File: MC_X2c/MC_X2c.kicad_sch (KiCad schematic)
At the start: 0 parts

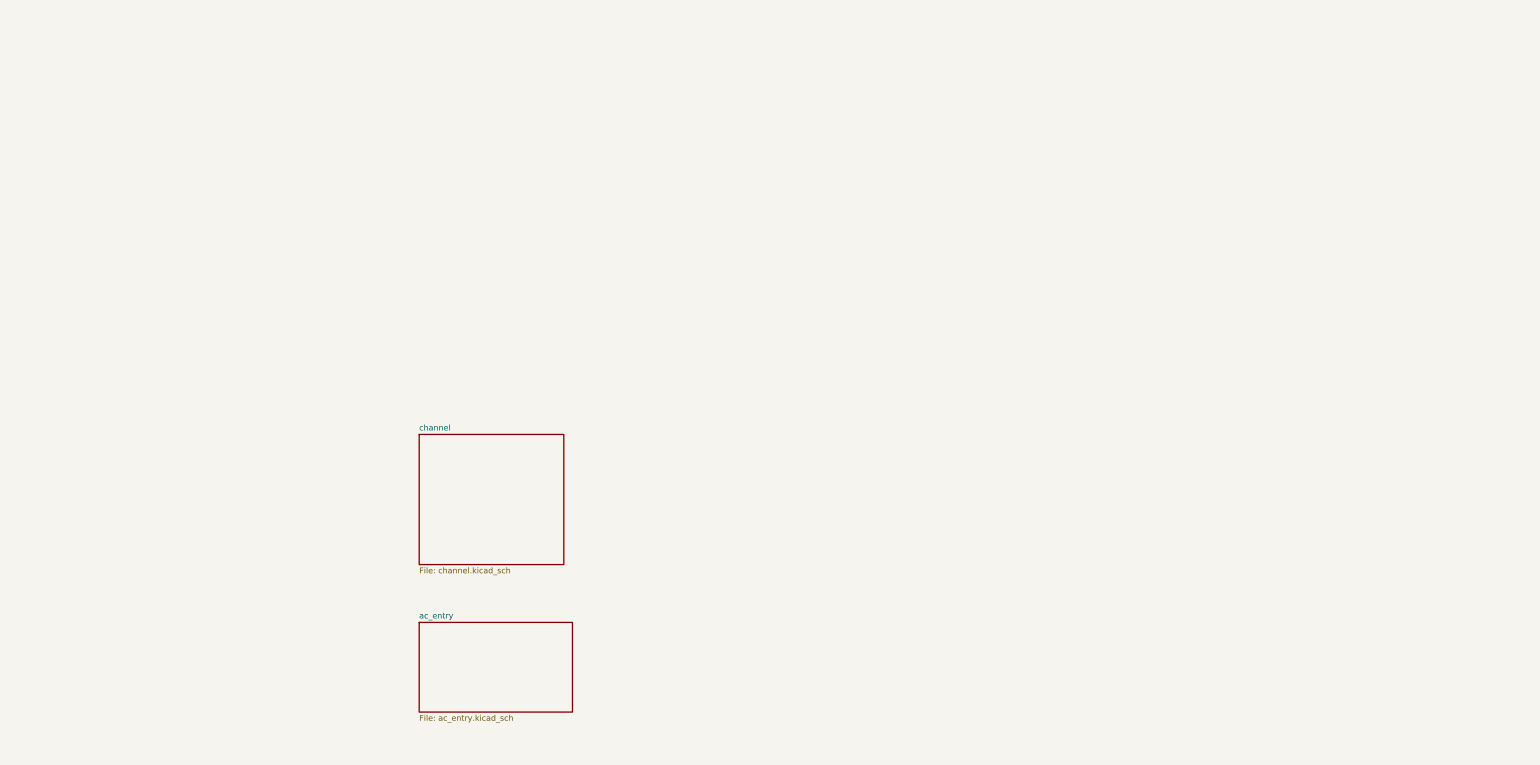
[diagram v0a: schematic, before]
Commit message: Working progress - migration to MAC
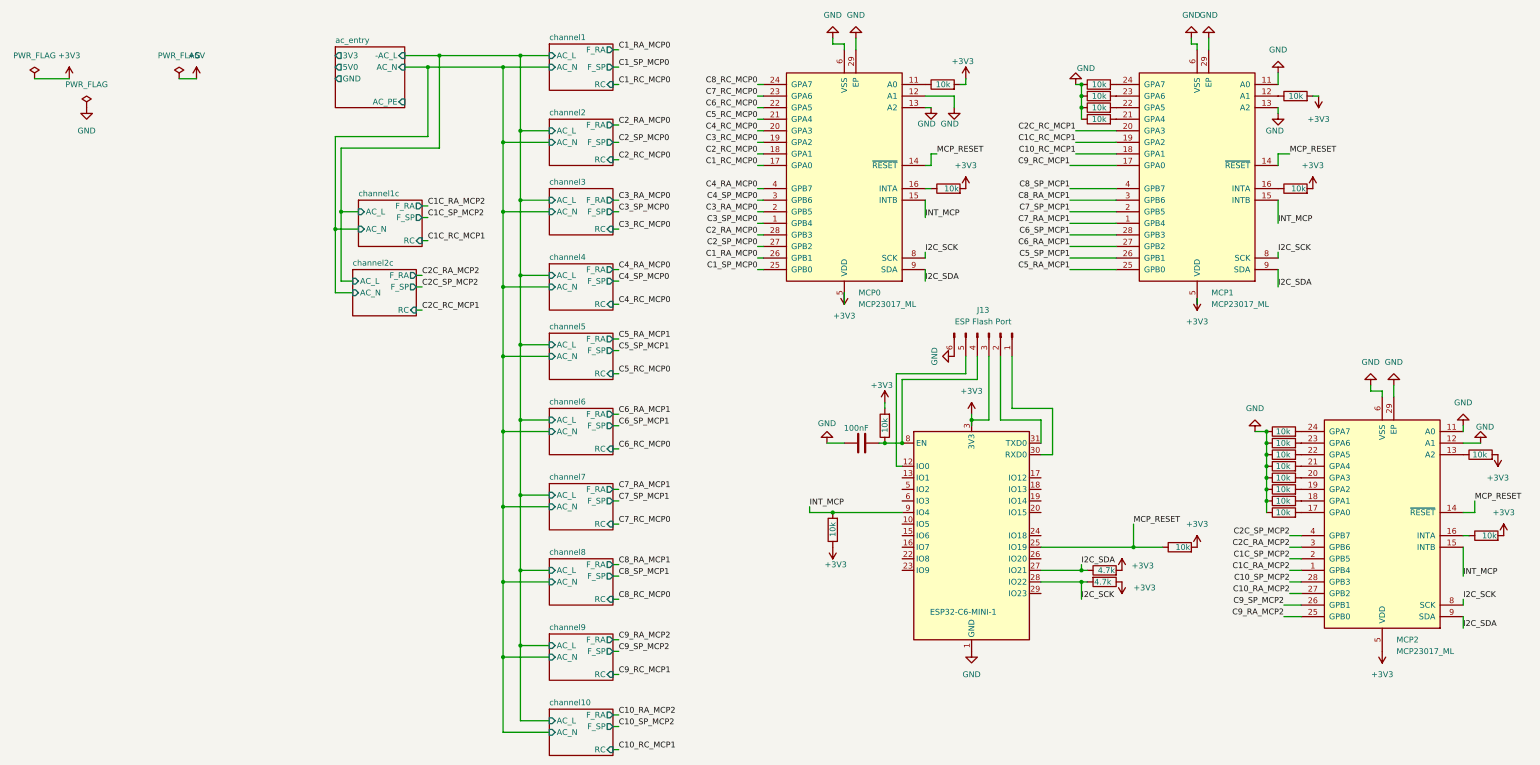
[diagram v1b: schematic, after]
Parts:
- added C34: 100nF, symbol Device:C
- added J13: ESP Flash Port, Connector_Harwin:Harwin_M20-89006xx_1x06_P2.54mm_Horizontal, symbol Connector:Conn_01x06_Pin
- added MCP0, MCP1, MCP2: MCP23017_ML, Package_DFN_QFN:QFN-28-1EP_6x6mm_P0.65mm_EP4.25x4.25mm, symbol Interface_Expansion:MCP23017_ML
- added R1, R102, R103, R104, R105, R106, R107, R108, R109, R110, R111, R112, R113, R114, R115, R116, R117, R118, R119, R4, R5: 10k, symbol Device:R
- added R2, R3: 4.7k, symbol Device:R
- added U1: ESP32-C6-MINI-1, RF_Module:ESP32-C6-MINI-1, symbol RF_Module:ESP32-C6-MINI-1
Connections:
- new net: MCP2.24 (GPA7), R109.2
- new net: MCP1.12 (A1), R4.1
- new net: J13.5 (Pin_5), U1.12 (IO0)
- new net: J13.1 (Pin_1), U1.30 (RXD0)
- new net: J13.2 (Pin_2), U1.31 (TXD0)
- new net: C34.2, J13.4 (Pin_4), R103.1, U1.8 (EN)
- new net: MCP1.24 (GPA7), R107.2
- new net: MCP2.18 (GPA1), R115.2
- new net: MCP1.16 (INTA), R119.1
- new net: MCP1.21 (GPA4), R108.2
- new net: MCP1.22 (GPA5), R106.2
- new net: MCP1.23 (GPA6), R105.2
- new net: MCP0.16 (INTA), R118.1
- new net: MCP2.21 (GPA4), R112.2
- new net: MCP2.16 (INTA), R117.1
- new net: MCP0.11 (A0), R1.1
- new net: MCP2.20 (GPA3), R113.2
- new net: MCP2.13 (A2), R5.1
- new net: MCP2.19 (GPA2), R114.2
- new net: MCP2.23 (GPA6), R110.2
- new net: MCP2.22 (GPA5), R111.2
- new net: MCP2.17 (GPA0), R116.2
- new net +3V3: J13.3 (Pin_3), MCP0.5 (VDD), MCP1.5 (VDD), MCP2.5 (VDD), R1.2, R102.2, R103.2, R104.1, R117.2, R118.2, R119.2, R2.2, R3.1, R4.2, R5.2, U1.3 (3V3)
- new net C10_RA_MCP2: MCP2.27 (GPB2)
- new net C10_RC_MCP1: MCP1.18 (GPA1)
- new net C10_SP_MCP2: MCP2.28 (GPB3)
- new net C1C_RA_MCP2: MCP2.1 (GPB4)
- new net C1C_RC_MCP1: MCP1.19 (GPA2)
- new net C1C_SP_MCP2: MCP2.2 (GPB5)
- new net C1_RA_MCP0: MCP0.26 (GPB1)
- new net C1_RC_MCP0: MCP0.17 (GPA0)
- new net C1_SP_MCP0: MCP0.25 (GPB0)
- new net C2C_RA_MCP2: MCP2.3 (GPB6)
- new net C2C_RC_MCP1: MCP1.20 (GPA3)
- new net C2C_SP_MCP2: MCP2.4 (GPB7)
- new net C2_RA_MCP0: MCP0.28 (GPB3)
- new net C2_RC_MCP0: MCP0.18 (GPA1)
- new net C2_SP_MCP0: MCP0.27 (GPB2)
- new net C3_RA_MCP0: MCP0.2 (GPB5)
- new net C3_RC_MCP0: MCP0.19 (GPA2)
- new net C3_SP_MCP0: MCP0.1 (GPB4)
- new net C4_RA_MCP0: MCP0.4 (GPB7)
- new net C4_RC_MCP0: MCP0.20 (GPA3)
- new net C4_SP_MCP0: MCP0.3 (GPB6)
- new net C5_RA_MCP1: MCP1.25 (GPB0)
- new net C5_RC_MCP0: MCP0.21 (GPA4)
- new net C5_SP_MCP1: MCP1.26 (GPB1)
- new net C6_RA_MCP1: MCP1.27 (GPB2)
- new net C6_RC_MCP0: MCP0.22 (GPA5)
- new net C6_SP_MCP1: MCP1.28 (GPB3)
- new net C7_RA_MCP1: MCP1.1 (GPB4)
- new net C7_RC_MCP0: MCP0.23 (GPA6)
- new net C7_SP_MCP1: MCP1.2 (GPB5)
- new net C8_RA_MCP1: MCP1.3 (GPB6)
- new net C8_RC_MCP0: MCP0.24 (GPA7)
- new net C8_SP_MCP1: MCP1.4 (GPB7)
- new net C9_RA_MCP2: MCP2.25 (GPB0)
- new net C9_RC_MCP1: MCP1.17 (GPA0)
- new net C9_SP_MCP2: MCP2.26 (GPB1)
- new net GND: C34.1, J13.6 (Pin_6), MCP0.12 (A1), MCP0.13 (A2), MCP0.29 (EP), MCP0.6 (VSS), MCP1.11 (A0), MCP1.13 (A2), MCP1.29 (EP), MCP1.6 (VSS), MCP2.11 (A0), MCP2.12 (A1), MCP2.29 (EP), MCP2.6 (VSS), R105.1, R106.1, R107.1, R108.1, R109.1, R110.1, R111.1, R112.1, R113.1, R114.1, R115.1, R116.1, U1.1 (GND), U1.11 (GND), U1.14 (GND), U1.2 (GND), U1.36 (GND), U1.37 (GND), U1.38 (GND), U1.39 (GND), U1.40 (GND), U1.41 (GND), U1.42 (GND), U1.43 (GND), U1.44 (GND), U1.45 (GND), U1.46 (GND), U1.47 (GND), U1.48 (GND), U1.49 (GND), U1.50 (GND), U1.51 (GND), U1.52 (GND), U1.53 (GND)
- new net I2C_SCK: MCP0.8 (SCK), MCP1.8 (SCK), MCP2.8 (SCK), R3.2, U1.28 (IO22)
- new net I2C_SDA: MCP0.9 (SDA), MCP1.9 (SDA), MCP2.9 (SDA), R2.1, U1.27 (IO21)
- new net INT_MCP: MCP0.15 (INTB), MCP1.15 (INTB), MCP2.15 (INTB), R104.2, U1.9 (IO4)
- new net MCP_RESET: MCP0.14 (~{RESET}), MCP1.14 (~{RESET}), MCP2.14 (~{RESET}), R102.1, U1.25 (IO19)
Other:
- sheet channel renamed channel1
- added sheet channel10 (channel.kicad_sch)
- added sheet channel1c (channel.kicad_sch)
- added sheet channel2 (channel.kicad_sch)
- added sheet channel2c (channel.kicad_sch)
- added sheet channel3 (channel.kicad_sch)
- added sheet channel4 (channel.kicad_sch)
- added sheet channel5 (channel.kicad_sch)
- added sheet channel6 (channel.kicad_sch)
- added sheet channel7 (channel.kicad_sch)
- added sheet channel8 (channel.kicad_sch)
- added sheet channel9 (channel.kicad_sch)
- sheet ac_entry ports: added 3V3, 5V0, AC_N, AC_PE, GND, ­AC_L; removed none
- sheet channel1 ports: added AC_L, AC_N, F_RA, F_SP, RC; removed none
- company: (none) -> Nelees
- title: (none) -> MC-X2c
